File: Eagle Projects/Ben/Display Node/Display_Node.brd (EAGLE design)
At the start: 93 x 90 mm, 90 parts, among them Q1 16MHz, Q3 16MHz, Q4 16MHz, Q5 16MHz, Q6 2N7002, Q7 2N7002, U1 ATMEGA328P_TQFP, U2 MCP2551, X1 5566-6, X2 5566-6

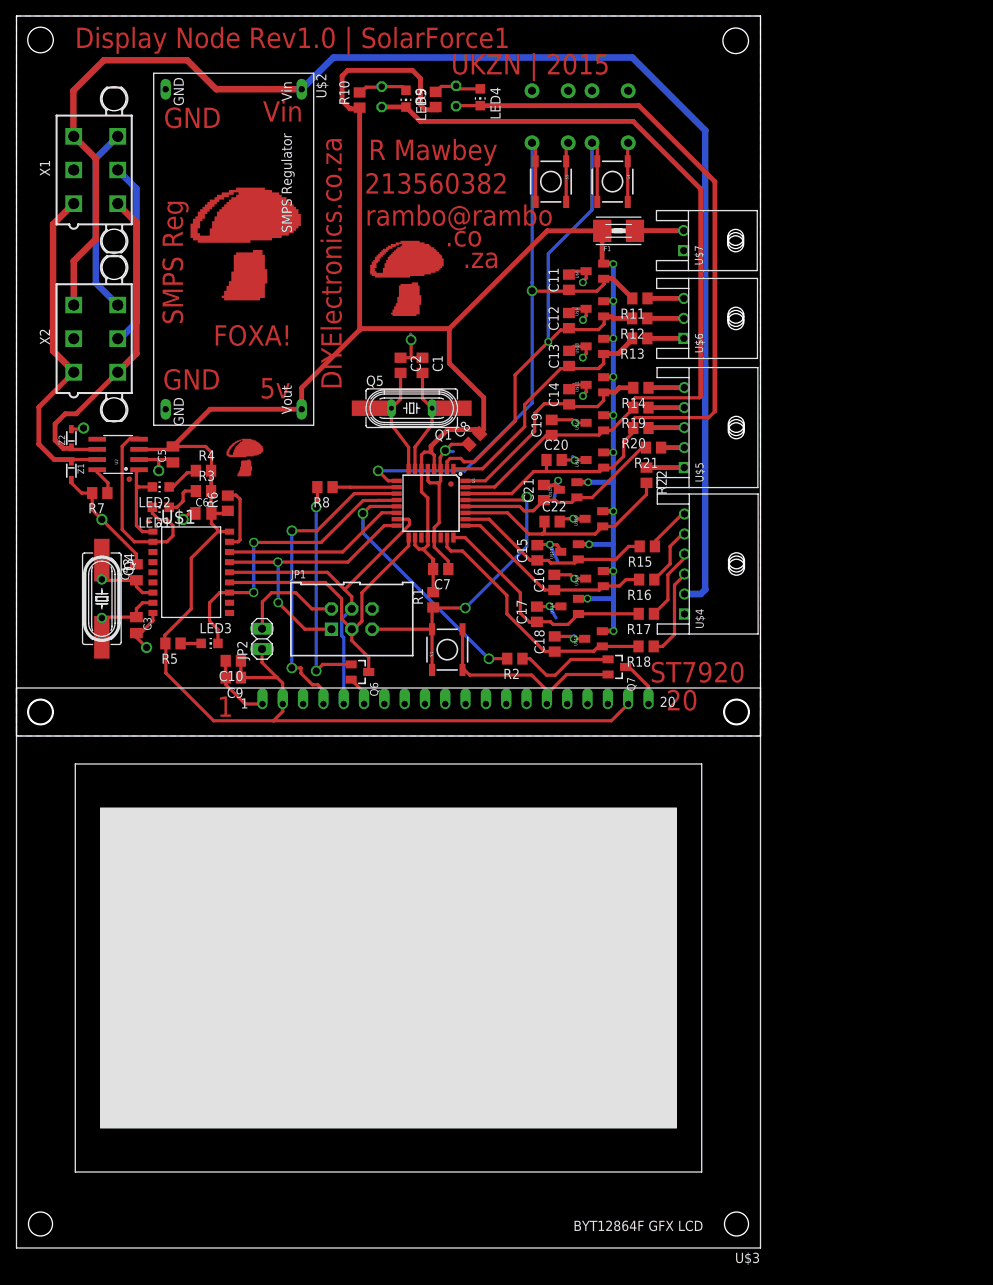
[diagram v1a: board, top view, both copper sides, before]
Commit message: Board Rework
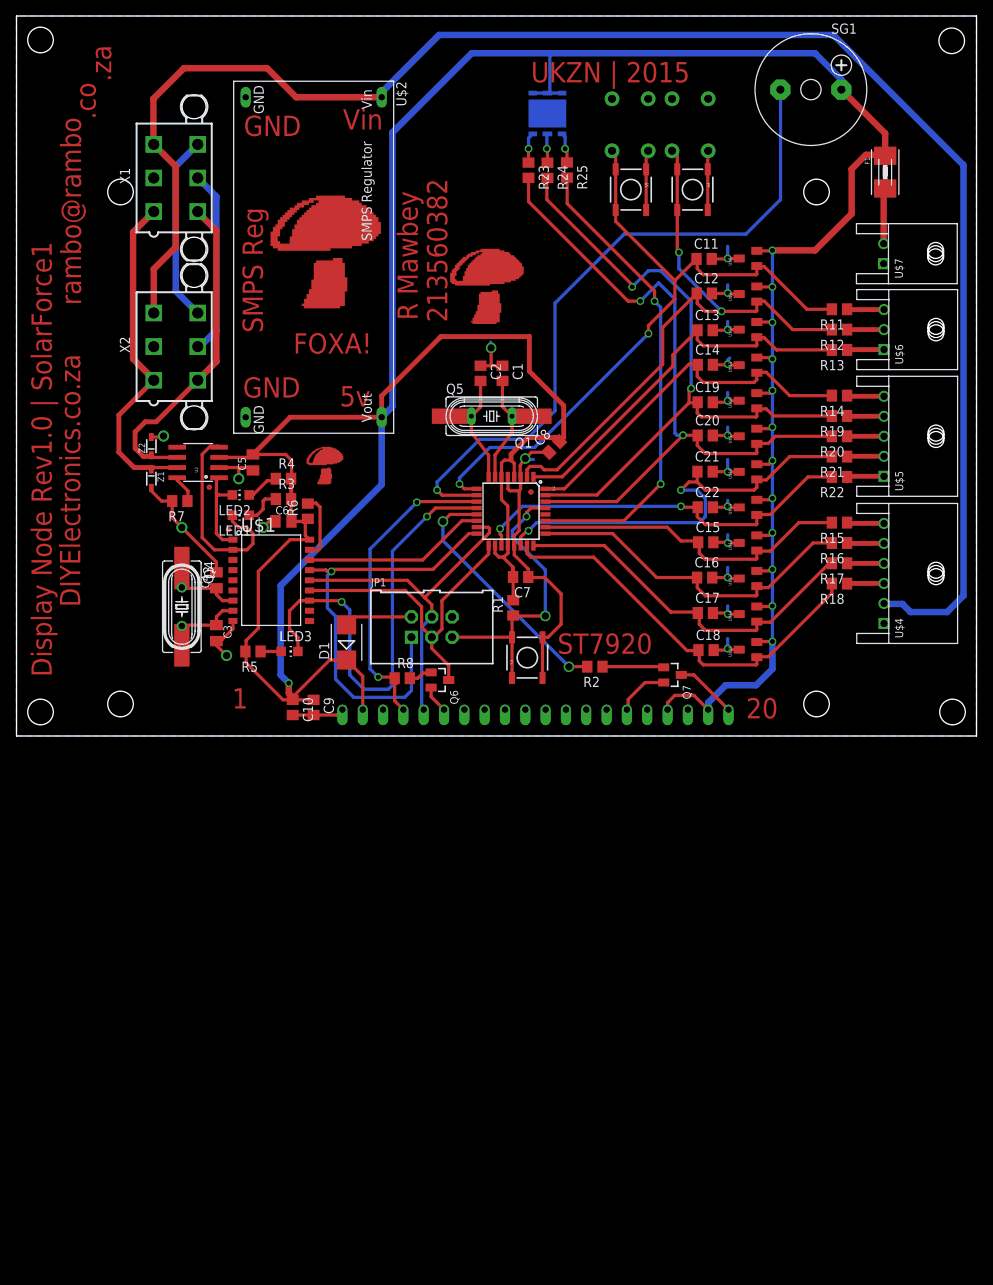
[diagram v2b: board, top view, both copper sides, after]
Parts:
- removed JP2: (no value), pinhead:1X02
- removed LED4, LED5: (no value), led:CHIP-LED0805
- removed LED6, LED7: (no value), led:LED5MM
- removed R10, R9: 1k, resistor:R0805
- added D1: (no value), diode:SMB
- added LED8: F50360, led:F50360
- added R23, R24, R25: 1k, resistor:R0805
- added SG1: F/CM12P, buzzer:F/CM12P
- moved F1 34.1 mm to (108.6, 70.5), turned to 270 degrees
- moved R8 25.8 mm to (48.2, 7.22), turned to 0 degrees
- moved R18 25.4 mm to (102.9, 19.1)
- moved U$7 25.1 mm to (114.9, 60.3)
- moved U$6 25.1 mm to (114.9, 50.8)
- moved R13 25.0 mm to (102.9, 48.3)
- moved R12 25.0 mm to (102.9, 50.8)
- moved U$5 25.0 mm to (114.9, 37.5)
- moved R11 25.0 mm to (102.9, 53.3)
- moved U$4 25.0 mm to (114.9, 20.3)
- moved R17 25.0 mm to (102.9, 21.6)
- moved R19 24.8 mm to (102.9, 40.0)
- moved R20 24.8 mm to (102.9, 37.5)
- moved R14 24.8 mm to (102.9, 42.5)
- moved R16 24.5 mm to (102.9, 24.1)
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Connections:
- removed net LCD_RST: U$3.P$4
- removed net N$13: LED4.A, LED7.A, R9.2
- removed net N$16: LED5.A, LED6.A, R10.2
- removed net SCKCNTRL: R8.1, U1.10
- new net LED3: R25.2, U1.27
- new net N$30: SG1.-, U1.10
- new net N$31: LED8.RC, R23.1
- new net N$32: LED8.GC, R24.1
- new net N$33: LED8.BC, R25.1
- new net N$36: U1.28
- net +5V: now also D1.C, LED8.BA, LED8.GA, LED8.RA, SG1.+, U$3.P$4; no longer JP2.1, R10.1, R9.1
- net A0: now also U1.19; no longer U1.27
- net A1: now also U1.22; no longer U1.28
- net LCD_CS: now also R8.1
- net LED1: now also R23.2; no longer LED4.C, LED7.K
- net LED2: now also R24.2; no longer LED5.C, LED6.K
- net N$10: now also D1.A; no longer JP2.2
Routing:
- net N$30: track 0.00 -> 85.4 mm, vias 0 -> 1
- net +5V: track 366.2 -> 439.0 mm, vias 12 -> 13
- net LED3: track 0.00 -> 59.5 mm, vias 0 -> 2
- net +12V: track 176.8 -> 208.8 mm
- net A1: track 26.3 -> 54.3 mm, vias 0 -> 2
- net N$12: track 27.7 -> 2.96 mm, vias 2 -> 0
- net A0: track 28.9 -> 49.6 mm, vias 0 -> 2
- net LED2: track 104.8 -> 84.3 mm, vias 0 -> 2
- net CANINT: track 37.9 -> 58.0 mm
- net CRUISE1: track 32.1 -> 51.1 mm
- net MISO: track 35.9 -> 54.5 mm, vias 2 -> 1
- net BTN1: track 28.0 -> 46.4 mm
- net CRUISE3: track 25.9 -> 43.3 mm
- net BTN2: track 32.0 -> 49.0 mm
- net CRUISE2: track 29.7 -> 46.5 mm
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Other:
- board size 93 x 90 mm -> 120 x 90 mm
